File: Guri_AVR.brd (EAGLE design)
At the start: 71 x 58.5 mm, 66 parts, among them IC1 7805, IC2 MEGA8-P, IC3 74LS74N, Q1 BC337, Q2 BC556, Q3 IRGB14C40L, Q5 BC548, X1 16.0

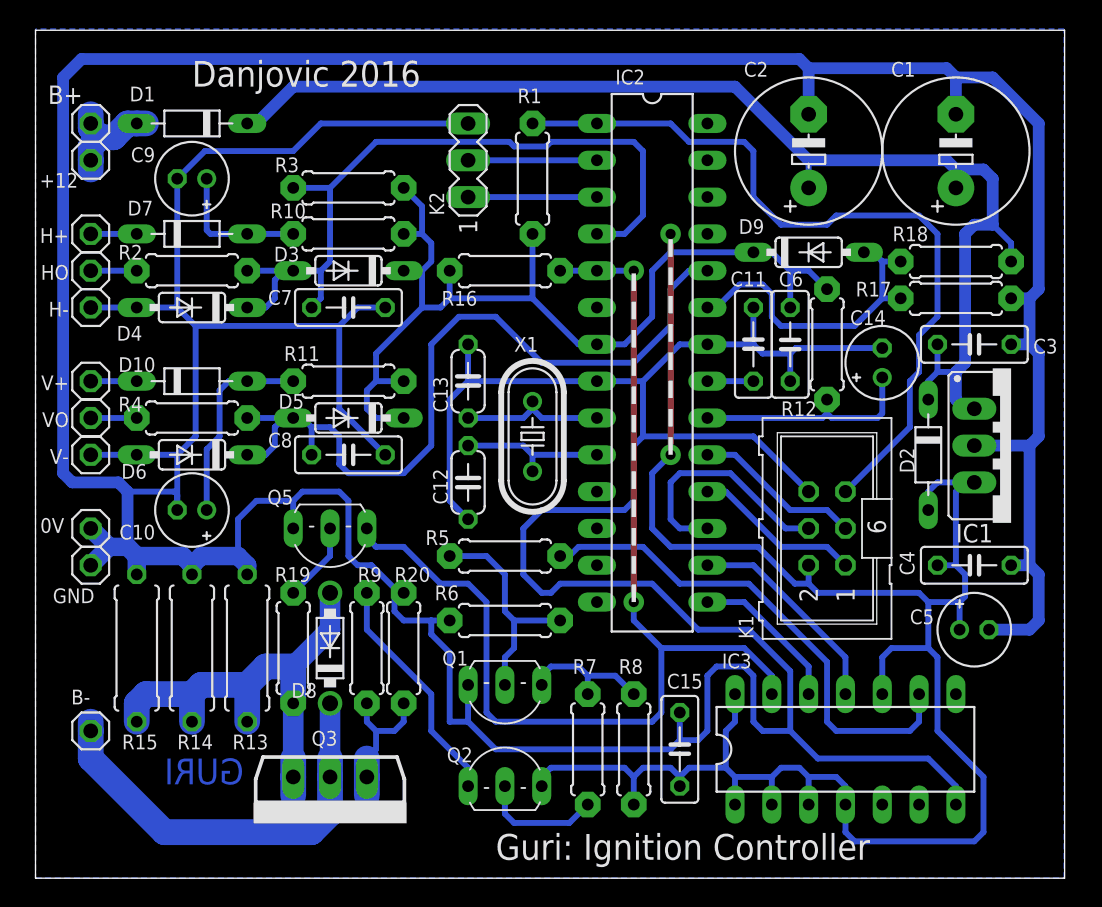
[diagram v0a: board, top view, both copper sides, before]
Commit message: New layout for preliminary board
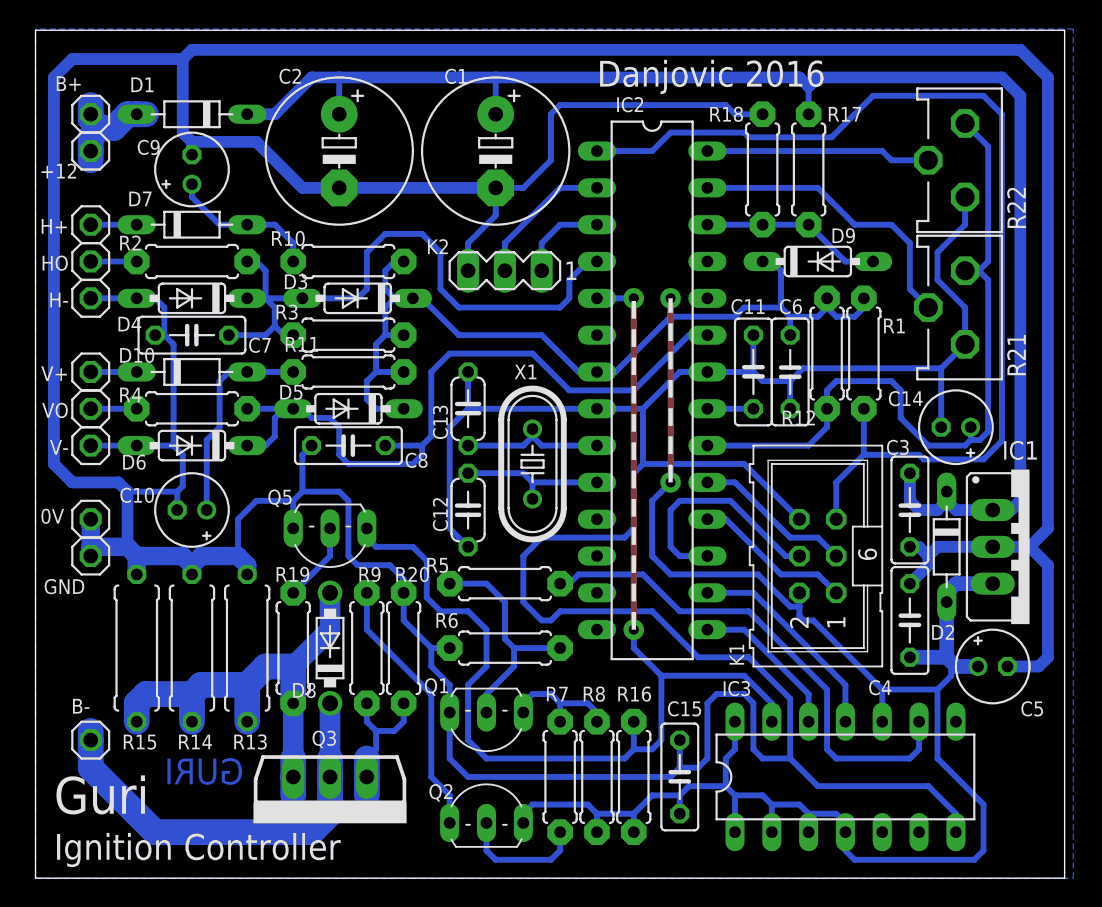
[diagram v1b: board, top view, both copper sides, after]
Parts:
- added R21, R22: 5K, pot:ECP10P
- moved R16 36.0 mm to (41.3, 6.99), turned to 270 degrees
- moved C2 32.4 mm to (21.0, 50.2), turned to 270 degrees
- moved C1 31.8 mm to (31.8, 50.2), turned to 270 degrees
- moved R1 25.8 mm to (57.1, 36.2), turned to 270 degrees
- moved R18 16.0 mm to (50.2, 48.9), turned to 90 degrees
- moved C3 12.3 mm to (60.3, 25.4), turned to 270 degrees
- moved R17 12.0 mm to (53.3, 48.9), turned to 270 degrees
- moved C7 11.0 mm to (10.8, 37.5), turned to 180 degrees
- moved R3 10.2 mm to (21.6, 37.5)
- moved K2 8.03 mm to (32.4, 41.9), turned to 180 degrees
- moved IC1 7.10 mm to (68.6, 22.9)
- moved C14 6.75 mm to (63.5, 31.1), turned to 180 degrees
- moved D2 6.48 mm to (62.9, 22.9)
- moved C4 5.85 mm to (60.3, 17.8), turned to 90 degrees
- moved R8 3.17 mm to (38.7, 6.99)
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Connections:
- new net N$16: IC2.27, R21.S
- new net N$17: IC2.28, R22.S
- net AVCC: now also R21.E, R22.E
- net GND: now also R21.A, R22.A
- net VACUUM: now also IC2.23; no longer IC2.24
- net VBAT: now also IC2.26; no longer IC2.23
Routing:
- net +12V: track 85.3 -> 128.9 mm
- net AVCC: track 15.9 -> 50.3 mm
- net GND: track 452.8 -> 483.7 mm
- net +5V: track 208.1 -> 187.5 mm
- net N$16: track 0.00 -> 20.5 mm
- net !RESET: track 53.9 -> 71.4 mm
- net N$17: track 0.00 -> 15.5 mm
- net VBAT: track 22.2 -> 12.5 mm
- net HALL: track 52.9 -> 43.7 mm
- net VACUUM: track 54.7 -> 50.1 mm
- net FF_RST: track 77.0 -> 80.9 mm
- net TXD: track 8.89 -> 6.24 mm
- net N$8: track 16.2 -> 18.2 mm
- net RXD: track 8.89 -> 9.83 mm
- net N$4: track 9.31 -> 8.41 mm
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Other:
- board text added: "Guri"
- board text added: "Ignition Controller"
- board text removed: "Guri: Ignition Controller"
